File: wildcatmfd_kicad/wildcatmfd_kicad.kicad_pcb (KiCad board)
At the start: 2 copper layers, 29 parts, among them SW1 SW_Push, SW10 SW_Push, SW11 SW_Push, SW12 SW_Push, SW13 SW_Push, SW14 SW_Push, SW15 SW_Push, SW16 SW_Push, SW17 SW_Push, SW18 SW_Push, SW19 SW_Push, SW2 SW_Push, SW20 SW_Push, SW21 SW_Push, SW22 SW_Push, SW23 SW_Push, SW24 SW_Push, SW25 SW_Push, SW26 SW_Push, SW27 SW_Push, SW28 SW_Push, SW3 SW_Push, SW4 SW_Push, SW5 SW_Push, SW6 SW_Push, SW7 SW_Push, SW8 SW_Push, SW9 SW_Push, U1 Teensy3.6

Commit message: Moved JOY_12 off of Pin 13
Pin 13 is the LED on the Teensy, not recommended to be used as an input
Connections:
- U1 pad 13: JOY_12 -> Net-(U1-Pad13)
- U1 pad 36: Net-(U1-Pad36) -> JOY_12

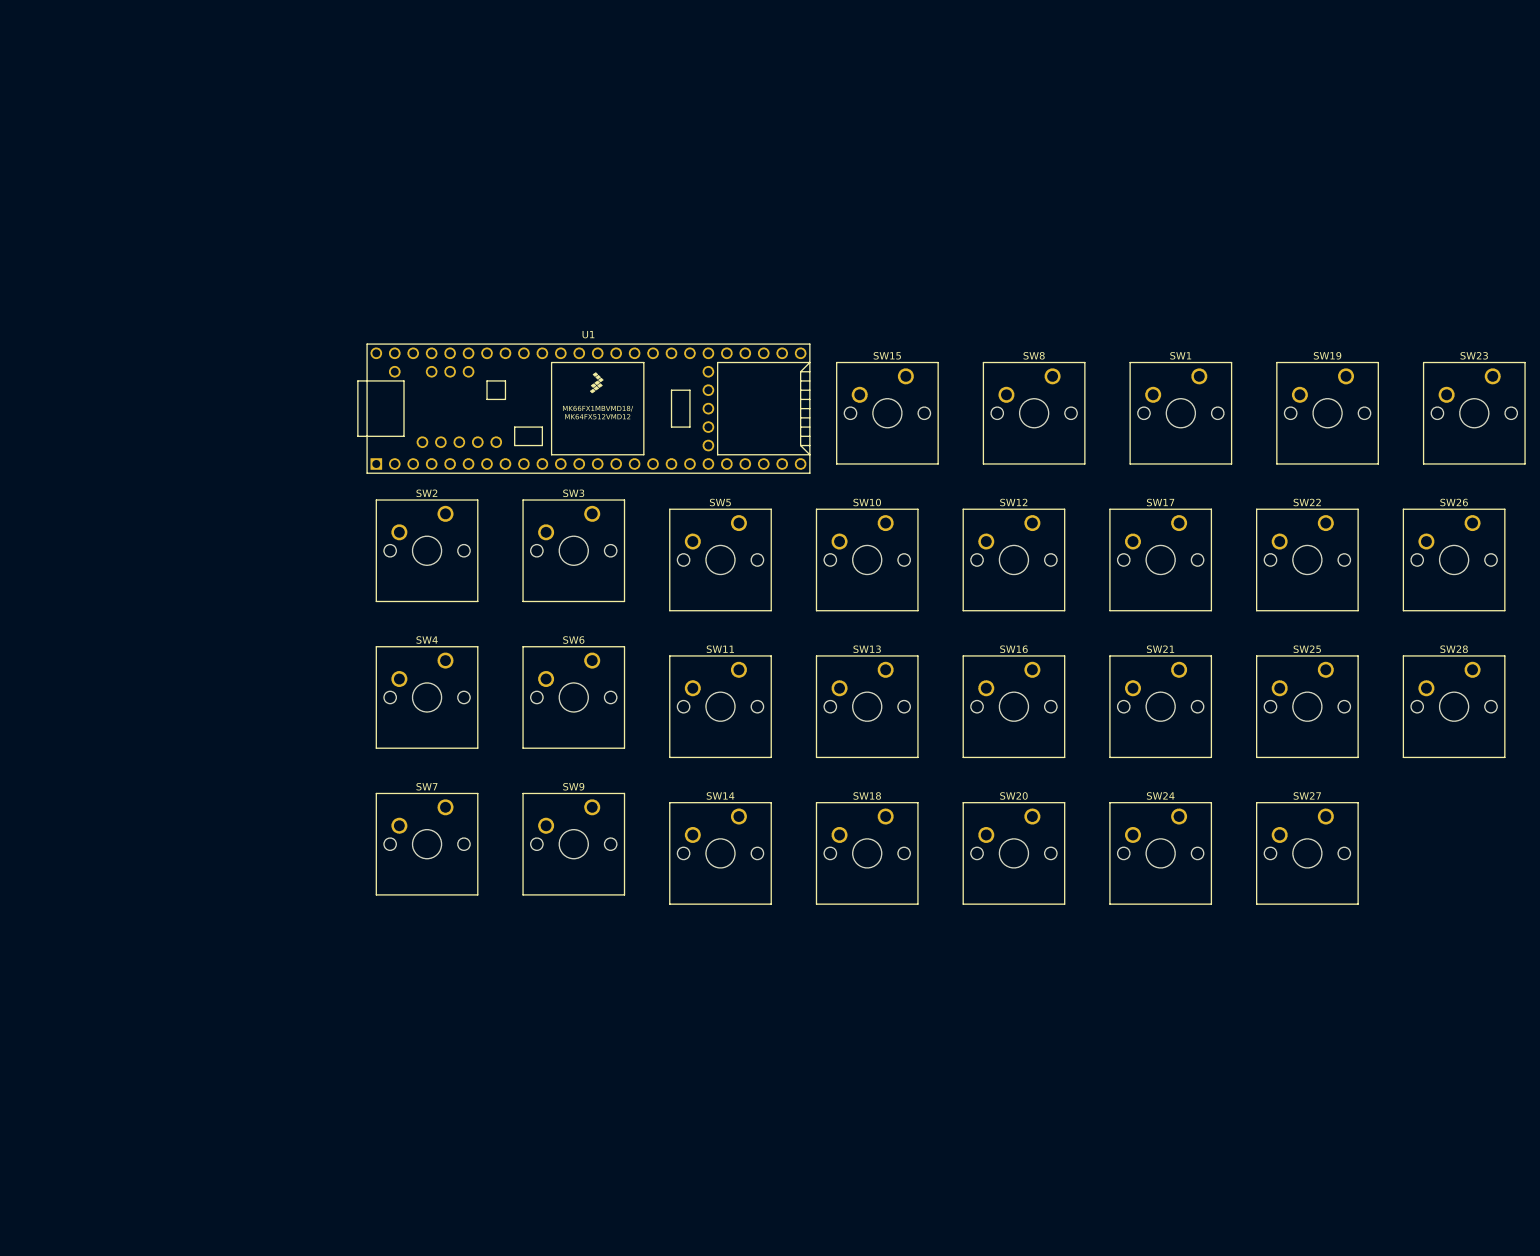
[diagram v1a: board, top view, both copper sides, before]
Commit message: More PCB work
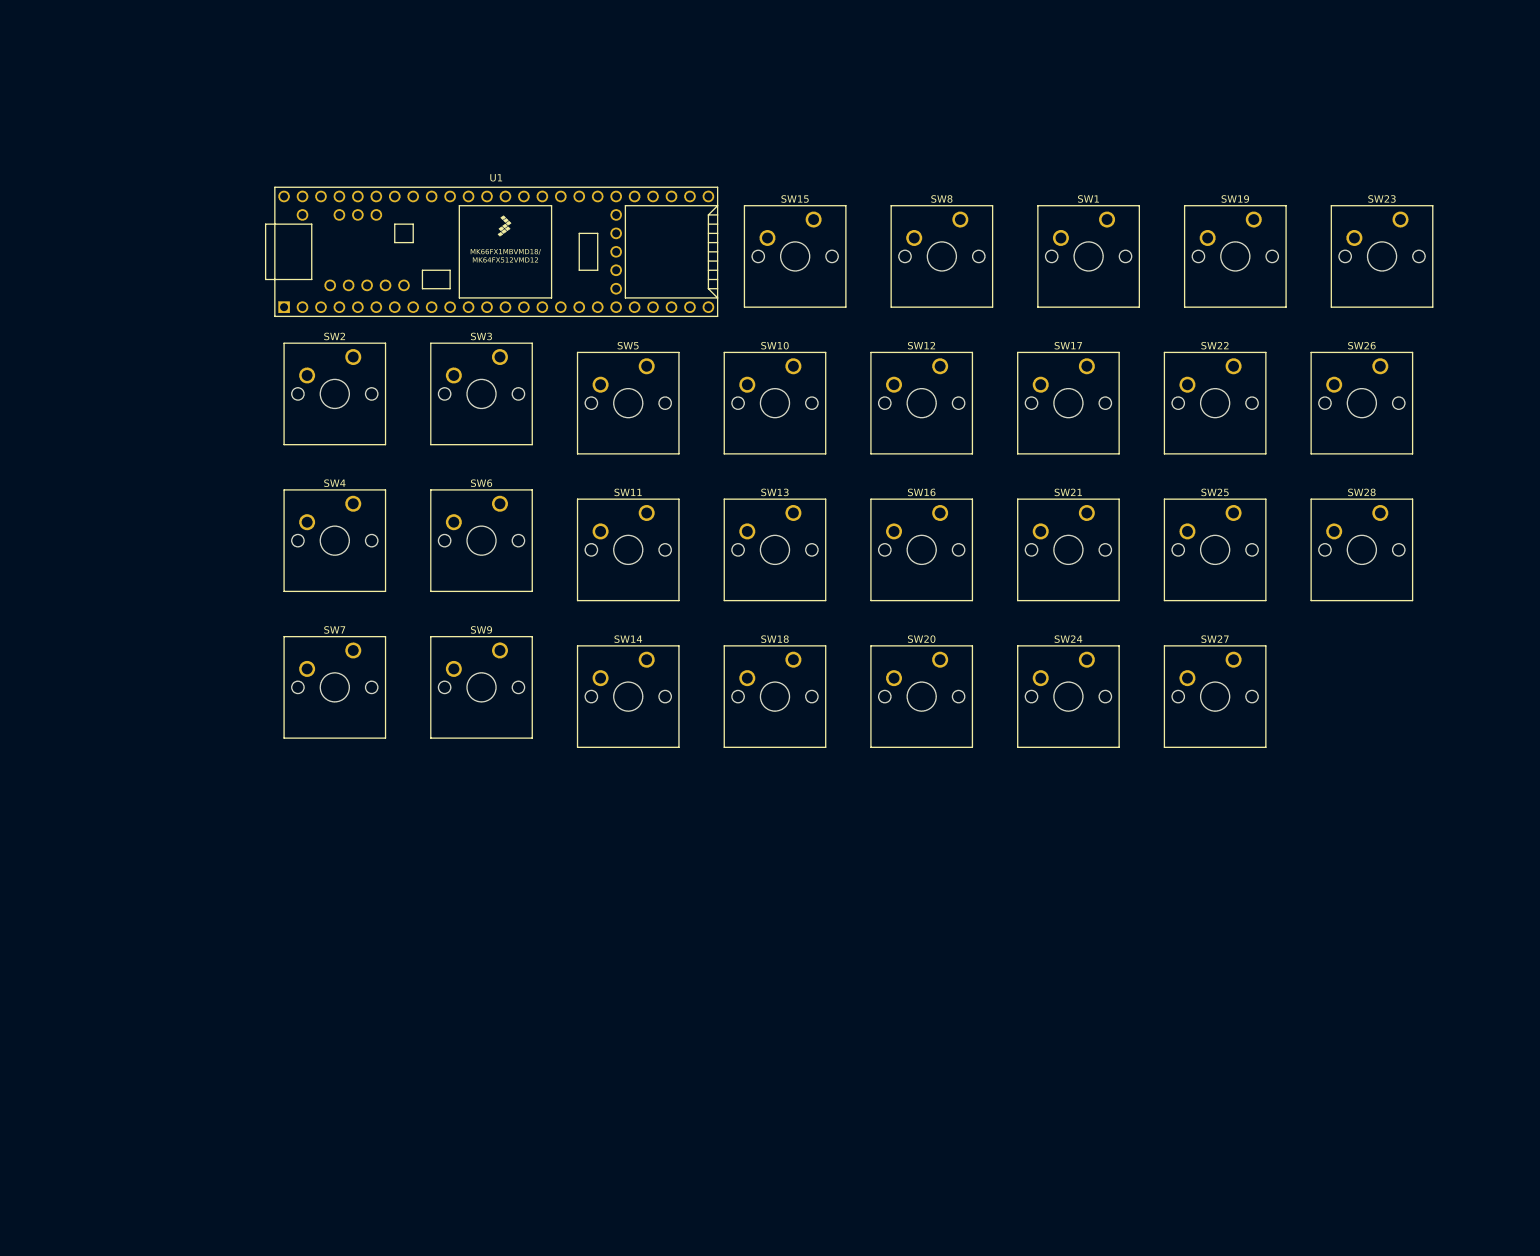
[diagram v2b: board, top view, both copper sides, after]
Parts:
- moved SW12 25.0 mm to (143.9, 64.9)
- moved SW16 25.0 mm to (143.9, 85.1)
- moved SW20 25.0 mm to (143.9, 105.3)
- moved SW22 25.0 mm to (184.3, 64.9)
- moved SW25 25.0 mm to (184.3, 85.1)
- moved SW27 25.0 mm to (184.3, 105.3)
- moved SW11 25.0 mm to (103.5, 85.1)
- moved SW14 25.0 mm to (103.5, 105.3)
- moved SW19 25.0 mm to (187.1, 44.7)
- moved SW3 25.0 mm to (83.3, 63.6)
- moved SW5 25.0 mm to (103.5, 64.9)
- moved SW6 25.0 mm to (83.3, 83.8)
- moved SW8 25.0 mm to (146.7, 44.7)
- moved SW10 25.0 mm to (123.7, 64.9)
- moved SW13 25.0 mm to (123.7, 85.1)
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
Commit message: Version 1.0 Complete
Will order PCBs!
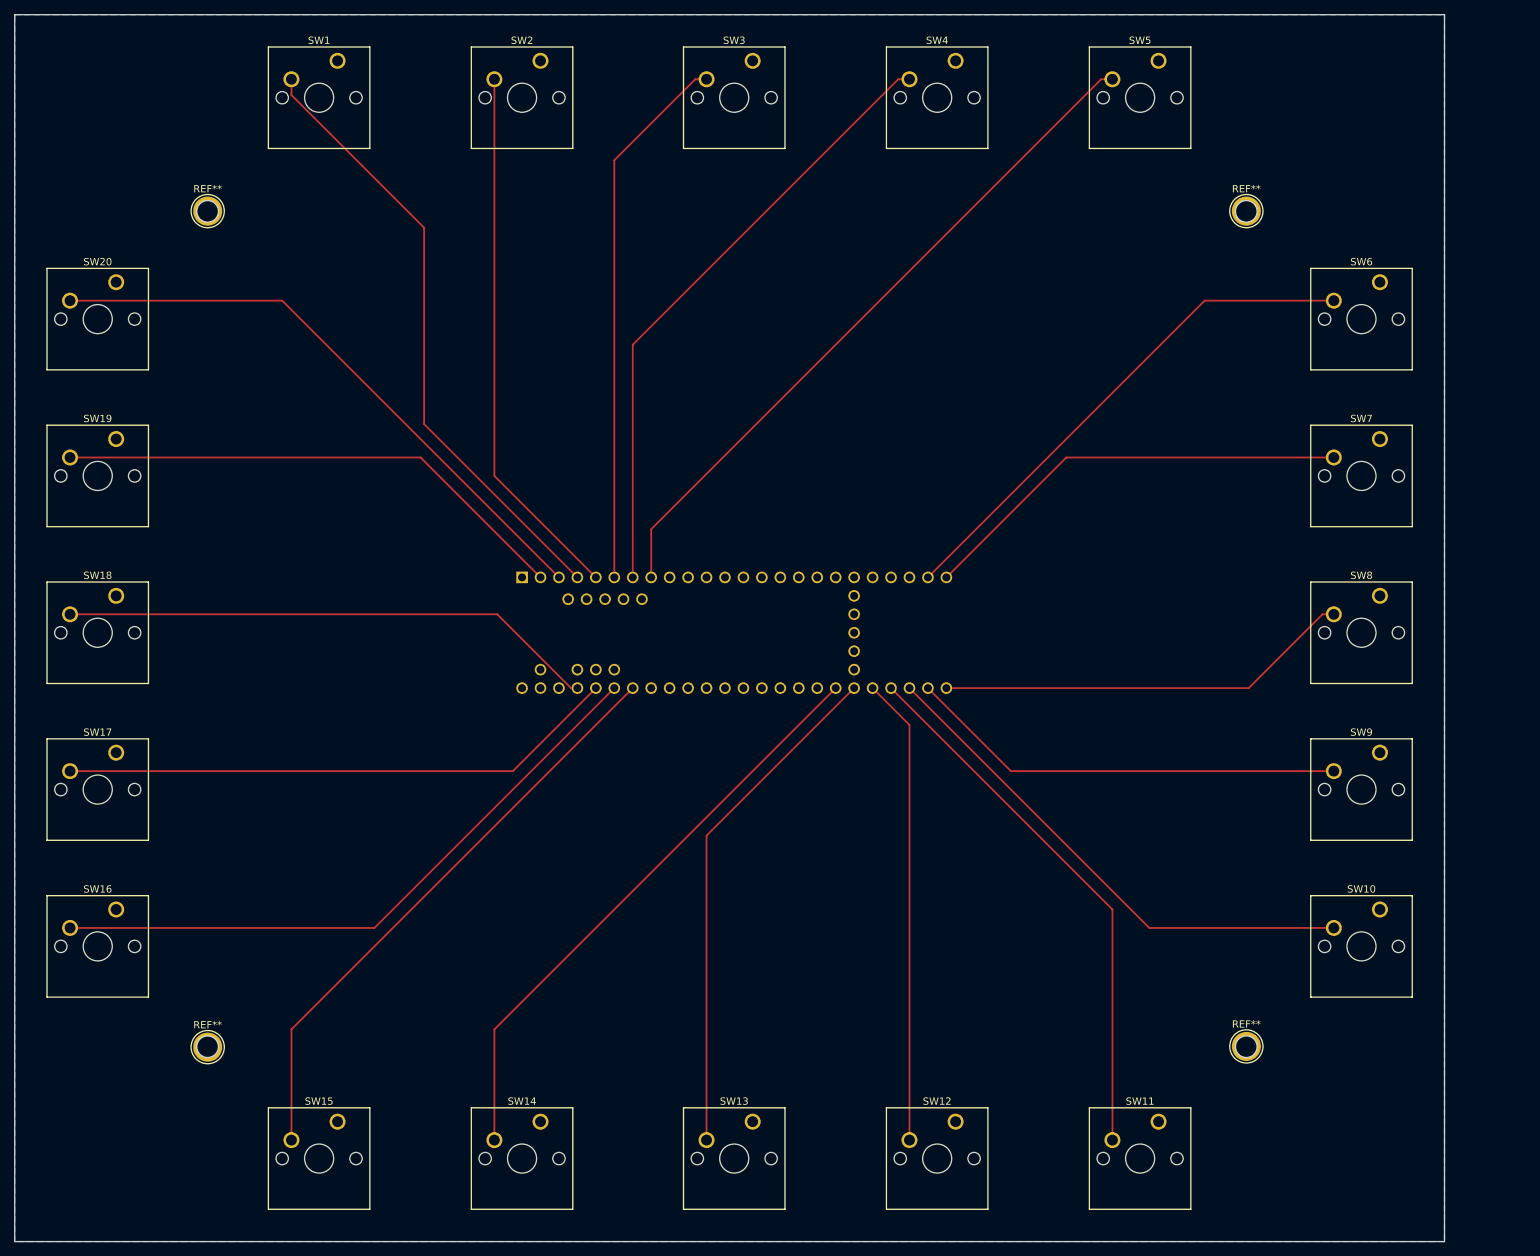
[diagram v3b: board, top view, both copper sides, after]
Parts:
- removed SW21, SW22, SW23, SW24, SW25, SW26, SW27, SW28: SW_Push, Button_Switch_Keyboard:SW_Cherry_MX_1.00u_PCB
- added REF**: TestPoint_Plated_Hole_D3.0mm, TestPoint:TestPoint_Plated_Hole_D3.0mm, F.Cu at (43.1, 158.7)
- added REF**: TestPoint_Plated_Hole_D3.0mm, TestPoint:TestPoint_Plated_Hole_D3.0mm, F.Cu at (186.1, 158.6)
- added REF**: TestPoint_Plated_Hole_D3.0mm, TestPoint:TestPoint_Plated_Hole_D3.0mm, F.Cu at (186.1, 43.5)
- added REF**: TestPoint_Plated_Hole_D3.0mm, TestPoint:TestPoint_Plated_Hole_D3.0mm, F.Cu at (43.1, 43.5)
- U1: moved to B.Cu
- moved SW19 159.5 mm to (30.5, 74.9)
- moved SW7 144.3 mm to (204.5, 74.9)
- moved SW17 143.8 mm to (30.5, 118.1)
- moved SW15 140.4 mm to (61.0, 168.9)
- moved SW16 125.9 mm to (30.5, 139.7)
- moved SW6 124.9 mm to (204.5, 53.3)
- moved SW20 124.8 mm to (30.5, 53.3)
- moved SW9 122.0 mm to (204.5, 118.1)
- moved SW10 110.1 mm to (204.5, 139.7)
- moved SW11 109.5 mm to (174.0, 168.9)
- moved SW1 108.2 mm to (61.0, 22.9)
- moved SW12 104.0 mm to (146.1, 168.9)
- moved SW4 102.9 mm to (146.1, 22.9)
- moved SW18 93.7 mm to (30.5, 96.5)
- moved SW13 84.0 mm to (118.1, 168.9)
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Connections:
- U1 pad 10: JOY_09 -> Net-(U1-Pad10)
- U1 pad 11: JOY_10 -> Net-(U1-Pad11)
- U1 pad 12: JOY_11 -> Net-(U1-Pad12)
- U1 pad 14: JOY_13 -> Net-(U1-Pad14)
- U1 pad 16: JOY_14 -> Net-(U1-Pad16)
- U1 pad 17: JOY_15 -> Net-(U1-Pad17)
- U1 pad 18: JOY_16 -> Net-(U1-Pad18)
- U1 pad 19: JOY_17 -> Net-(U1-Pad19)
- U1 pad 2: JOY_01 -> JOY_19
- U1 pad 20: JOY_18 -> Net-(U1-Pad20)
- U1 pad 21: JOY_19 -> Net-(U1-Pad21)
- U1 pad 22: JOY_20 -> Net-(U1-Pad22)
- U1 pad 23: JOY_21 -> JOY_06
- U1 pad 24: JOY_22 -> JOY_07
- U1 pad 3: JOY_02 -> JOY_20
- U1 pad 30: JOY_23 -> JOY_08
- U1 pad 31: JOY_24 -> JOY_09
- U1 pad 32: JOY_25 -> JOY_10
- U1 pad 33: JOY_26 -> JOY_11
- U1 pad 34: JOY_27 -> JOY_12
- U1 pad 35: JOY_28 -> JOY_13
- U1 pad 36: JOY_12 -> JOY_14
- U1 pad 4: JOY_03 -> JOY_01
- U1 pad 47: Net-(U1-Pad47) -> JOY_15
- U1 pad 48: Net-(U1-Pad48) -> JOY_16
- U1 pad 49: Net-(U1-Pad49) -> JOY_17
- U1 pad 5: JOY_04 -> JOY_02
- U1 pad 50: Net-(U1-Pad50) -> JOY_18
- U1 pad 6: JOY_05 -> JOY_03
- U1 pad 7: JOY_06 -> JOY_04
- U1 pad 8: JOY_07 -> JOY_05
- U1 pad 9: JOY_08 -> Net-(U1-Pad9)
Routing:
- net JOY_05: track 0.00 -> 95.8 mm
- net JOY_16: track 0.00 -> 88.6 mm
- net JOY_04: track 0.00 -> 85.3 mm
- net JOY_01: track 0.00 -> 84.9 mm
- net JOY_20: track 0.00 -> 83.1 mm
- net JOY_15: track 0.00 -> 81.7 mm
- net JOY_14: track 0.00 -> 81.7 mm
- net JOY_17: track 0.00 -> 77.1 mm
- net JOY_11: track 0.00 -> 74.9 mm
- net JOY_03: track 0.00 -> 74.8 mm
- net JOY_02: track 0.00 -> 74.4 mm
- net JOY_18: track 0.00 -> 74.1 mm
- net JOY_10: track 0.00 -> 72.1 mm
- net JOY_06: track 0.00 -> 71.7 mm
- net JOY_19: track 0.00 -> 71.6 mm
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- added copper zone on B.Cu, net GND
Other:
- board outline added: 196.9 x 168.9 mm
